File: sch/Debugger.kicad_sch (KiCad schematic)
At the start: 33 parts, among them J3 Conn_ARM_SWD_TagConnect_TC203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, Q1 Q_NMOS_GSD, U10 TPS22991, U12 TMUX1511RSVR, U6 TXU0204RUTR, U7 nRF52833-QDXX, U8 TXU0101DRYR, Y2 32MHz, 10pF

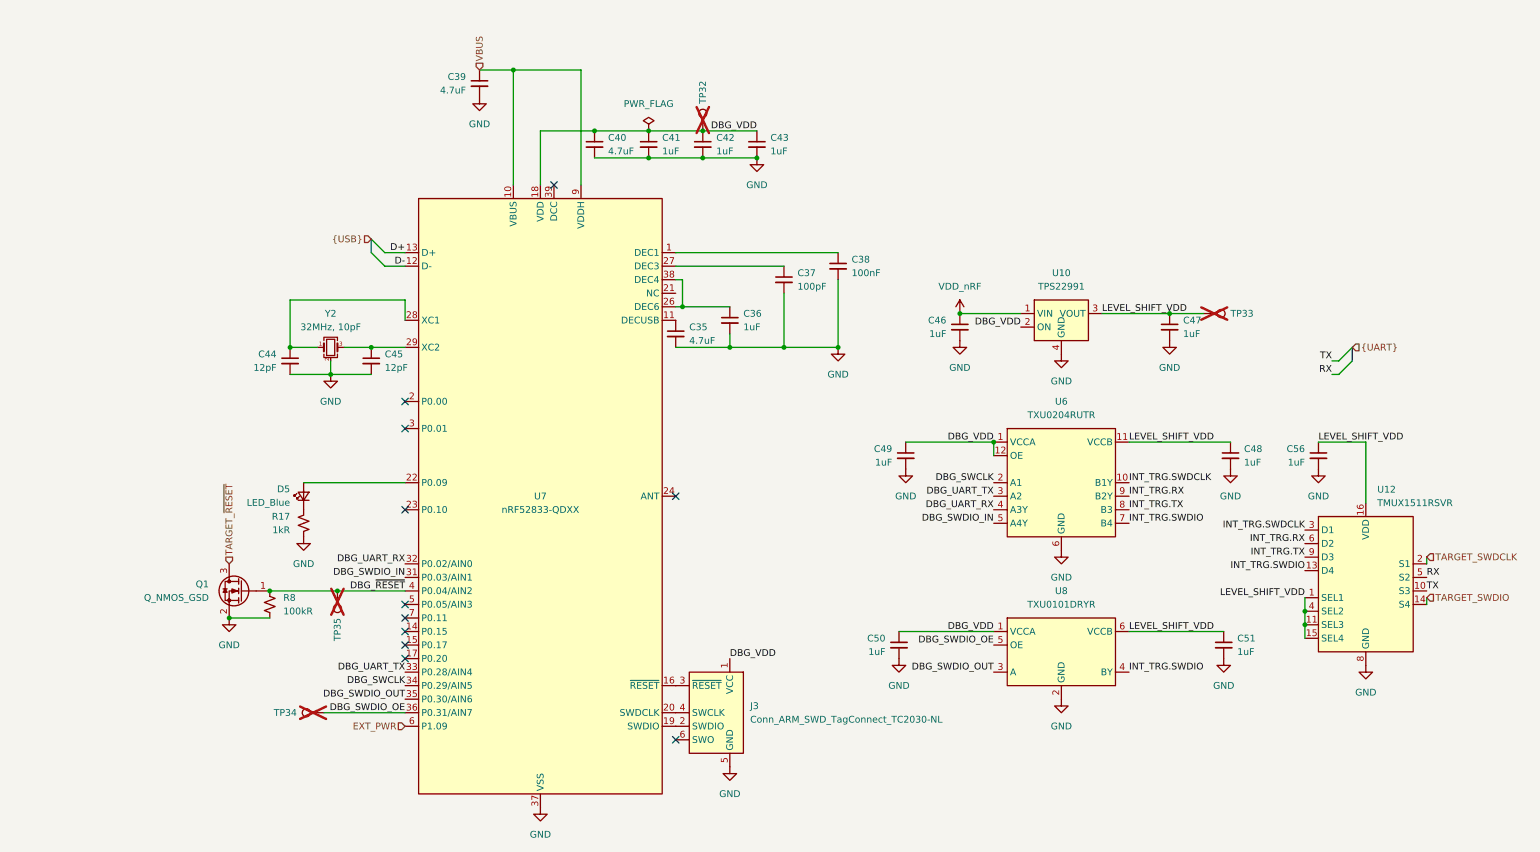
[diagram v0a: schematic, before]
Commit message: Updates for V2
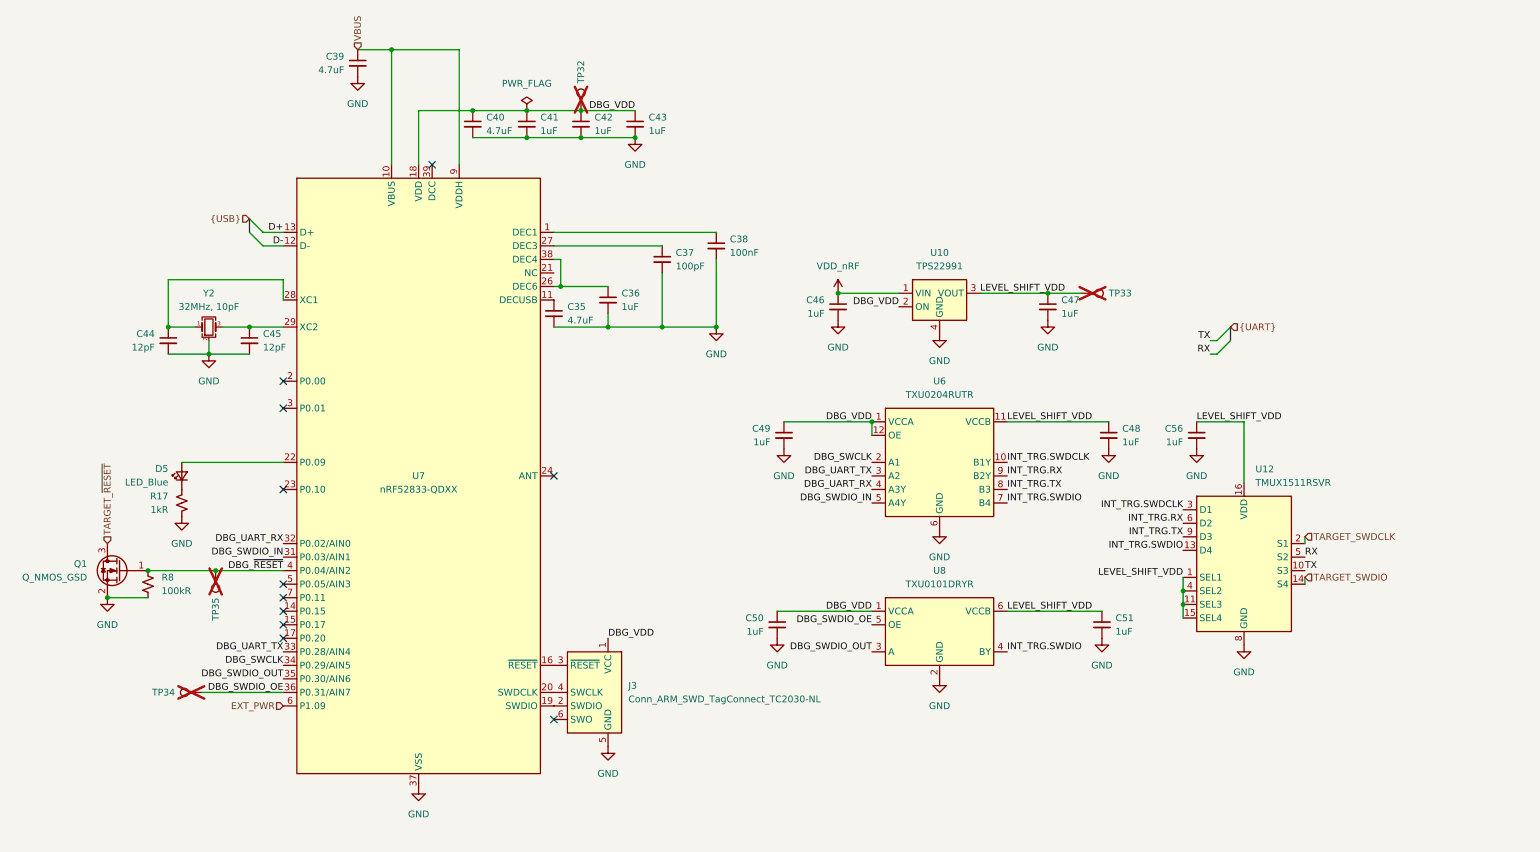
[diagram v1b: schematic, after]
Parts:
- Y2: LCSC C383840 -> C54427949
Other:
- moved on the sheet: C35, C36, C37, C38, C39, C40, C41, C42, C43, C44, C45, C46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
